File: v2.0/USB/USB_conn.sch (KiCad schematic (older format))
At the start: 11 parts, among them J1 Conn_01x10, J10 Conn_01x01, J11 Conn_01x01, J2 Conn_01x01, J3 Conn_01x01, J4 Conn_01x01, J5 Conn_01x01, J6 Conn_01x01, J7 Conn_01x01, J8 Conn_01x01, J9 Conn_01x01

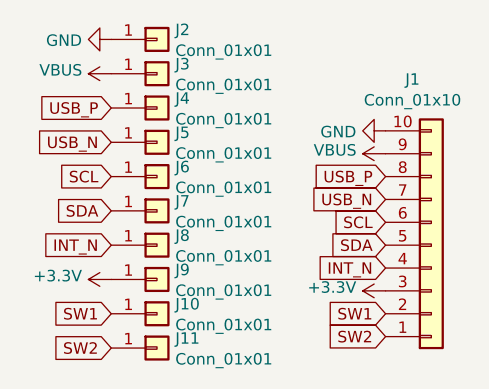
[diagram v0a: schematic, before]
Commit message: updated files
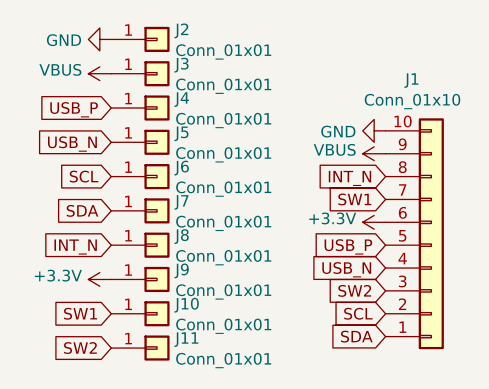
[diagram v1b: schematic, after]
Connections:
- net +3V3: now also J1.6 (Pin_6); no longer J1.3 (Pin_3)
- net INT_N: now also J1.8 (Pin_8); no longer J1.4 (Pin_4)
- net SCL: now also J1.2 (Pin_2); no longer J1.6 (Pin_6)
- net SDA: now also J1.1 (Pin_1); no longer J1.5 (Pin_5)
- net SW1: now also J1.7 (Pin_7); no longer J1.2 (Pin_2)
- net SW2: now also J1.3 (Pin_3); no longer J1.1 (Pin_1)
- net USB_N: now also J1.4 (Pin_4); no longer J1.7 (Pin_7)
- net USB_P: now also J1.5 (Pin_5); no longer J1.8 (Pin_8)
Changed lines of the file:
@@
 L power:+3.3V #PWR0103
 U 1 1 5E94BB3A
-P 7500 3250
-F 0 "#PWR0103" H 7500 3100 50  0001 C CNN
-F 1 "+3.3V" V 7515 3378 50  0000 L CNN
-F 2 "" H 7500 3250 50  0001 C CNN
-F 3 "" H 7500 3250 50  0001 C CNN
-	1    7500 3250
+P 7500 2950
+F 0 "#PWR0103" H 7500 2800 50  0001 C CNN
+F 1 "+3.3V" V 7515 3078 50  0000 L CNN
+F 2 "" H 7500 2950 50  0001 C CNN
+F 3 "" H 7500 2950 50  0001 C CNN
+	1    7500 2950
 	0    -1   -1   0
 $EndComp
+Text GLabel 7500 2850 0    50   Input ~ 0
+SW1
+Text GLabel 7500 3250 0    50   Input ~ 0
+SW2
+Text GLabel 7500 2750 0    50   Input ~ 0
+INT_N
+Text GLabel 7500 3450 0    50   Input ~ 0
+SDA
 Text GLabel 7500 3350 0    50   Input ~ 0
-SW1
-Text GLabel 7500 3450 0    50   Input ~ 0
-SW2
+SCL
+Text GLabel 7500 3050 0    50   Input ~ 0
+USB_P
 Text GLabel 7500 3150 0    50   Input ~ 0
-INT_N
-Text GLabel 7500 3050 0    50   Input ~ 0
-SDA
-Text GLabel 7500 2950 0    50   Input ~ 0
-SCL
-Text GLabel 7500 2750 0    50   Input ~ 0
-USB_P
-Text GLabel 7500 2850 0    50   Input ~ 0
 USB_N
 $Comp
